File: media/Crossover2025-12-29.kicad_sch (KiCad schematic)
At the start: 11 parts, among them J1 GPIO, J2 Qwiic Right Angle, J3 Conn_01x04_Female, J4 Conn_01x03_Pin, J5 Conn_01x08_Socket, J6 Conn_01x02_Pin, J7 Screw_Terminal_01x02, Q1 2N4124

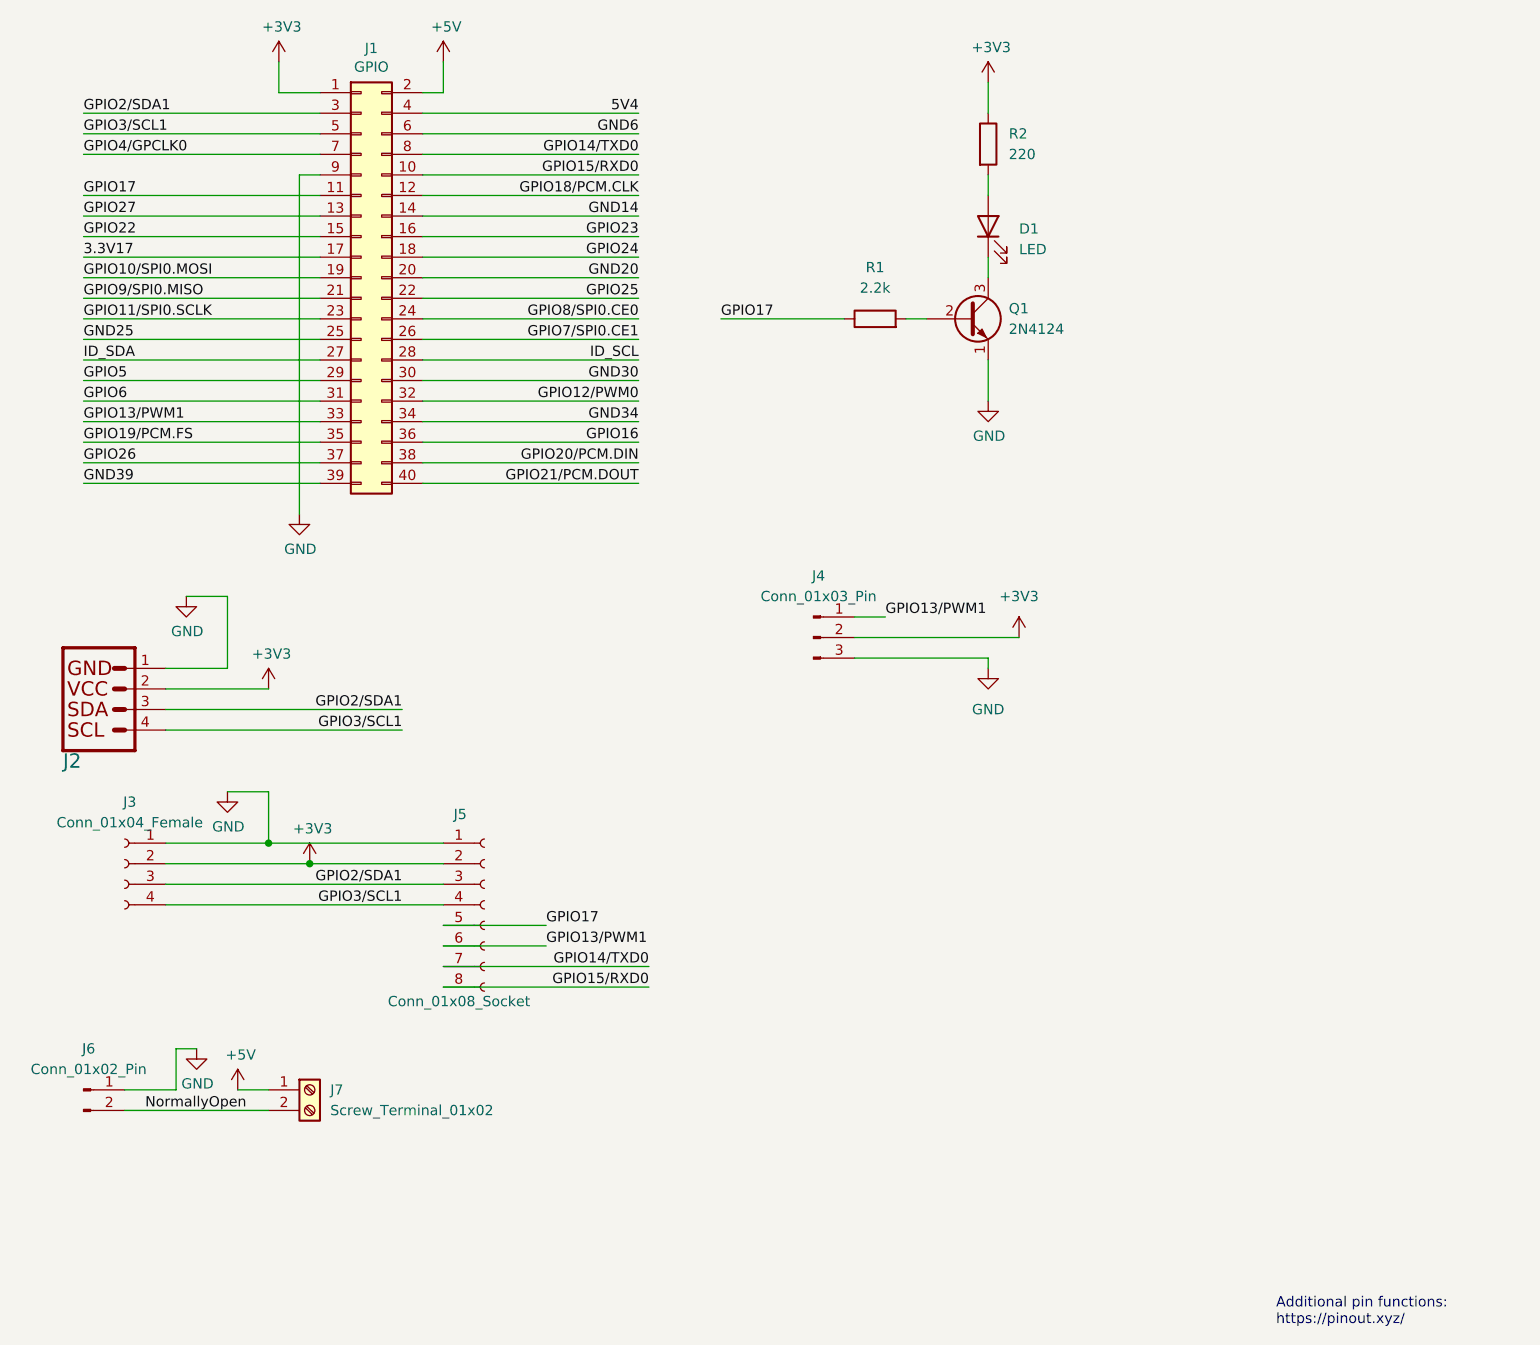
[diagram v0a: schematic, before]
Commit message: Add files via upload
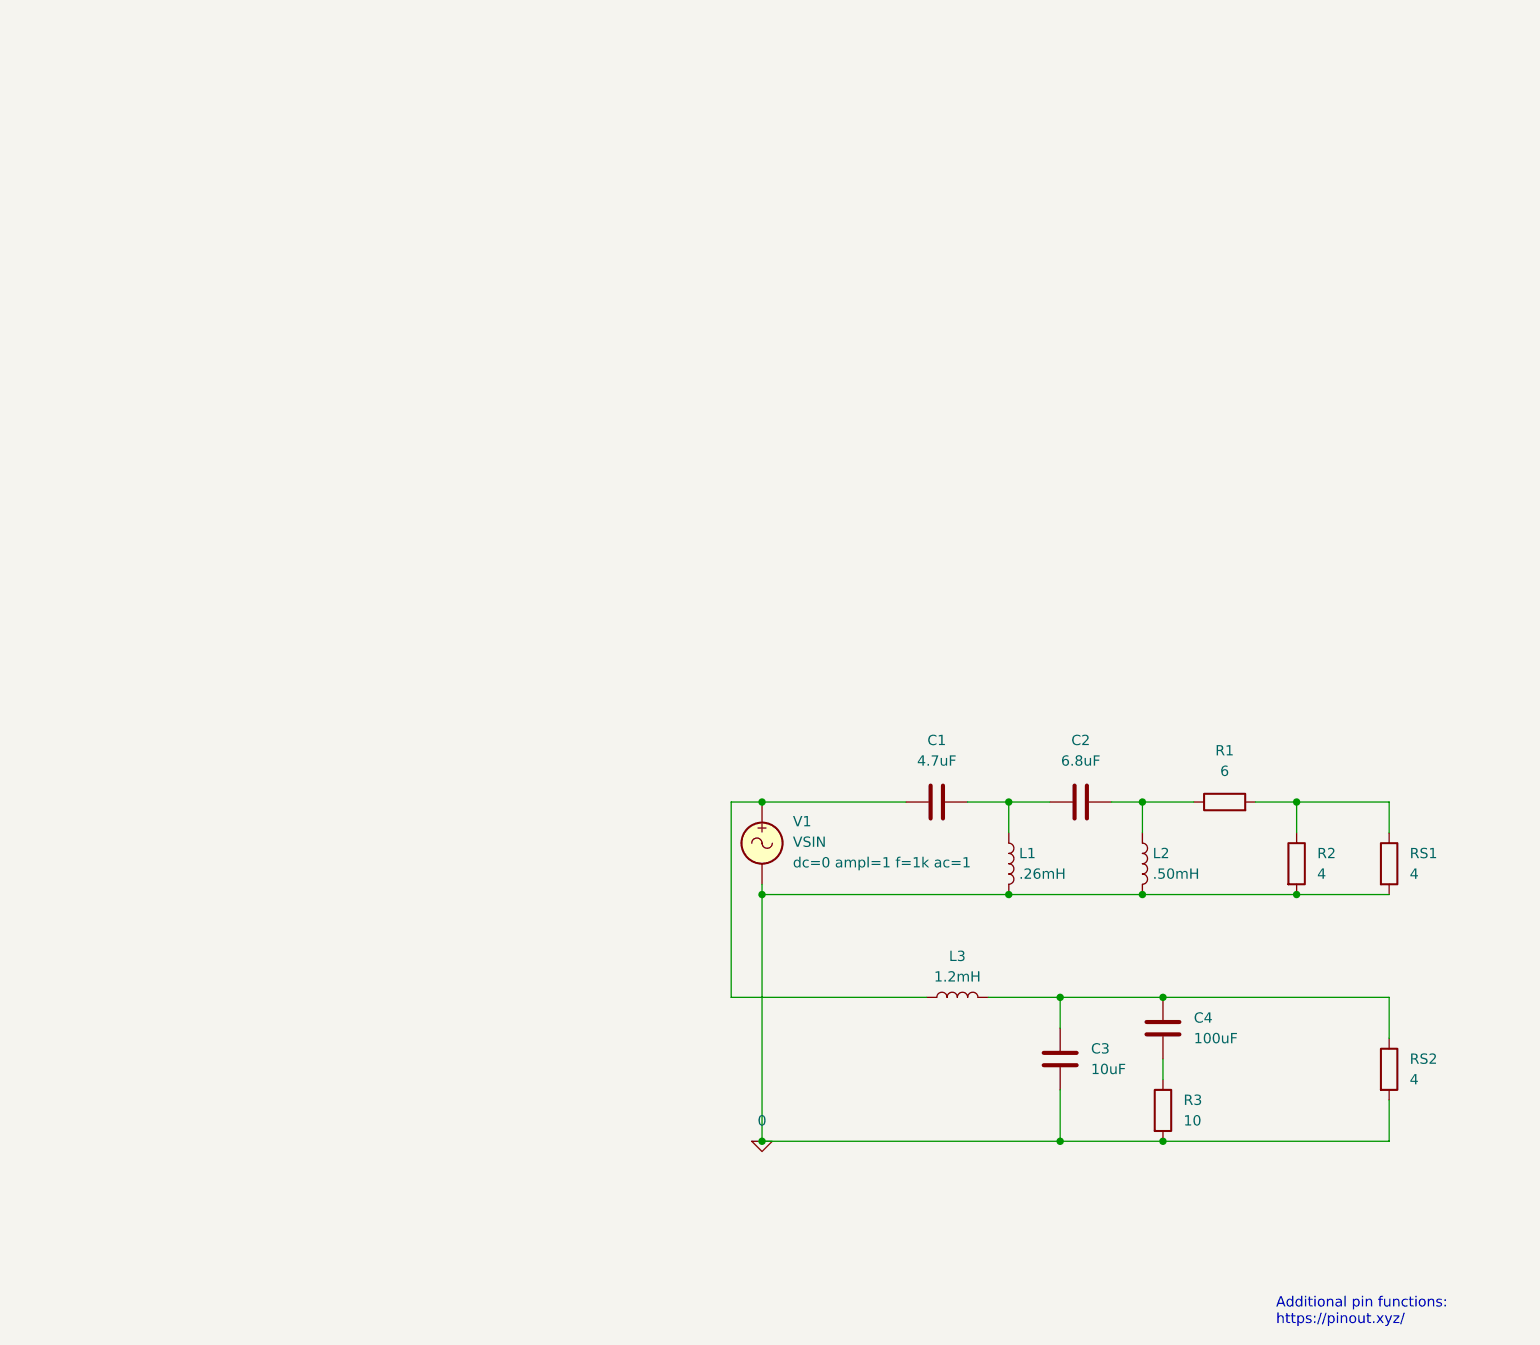
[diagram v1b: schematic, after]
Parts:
- removed D1: LED, LED_THT:LED_D5.0mm_Horizontal_O1.27mm_Z3.0mm, symbol Device:LED
- removed J1: GPIO, Connector_PinSocket_2.54mm:PinSocket_2x20_P2.54mm_Vertical, symbol Connector_Generic:Conn_02x20_Odd_Even
- removed J2: Qwiic Right Angle, Connector_PinSocket_2.00mm:PinSocket_1x04_P2.00mm_Horizontal, symbol Qwiic_pHat_for_Raspberry_Pi_v30-eagle-import:I2C_STANDARDQWIIC
- removed J3: Conn_01x04_Female, Connector_PinSocket_2.54mm:PinSocket_1x04_P2.54mm_Horizontal, symbol Connector:Conn_01x04_Female
- removed J4: Conn_01x03_Pin, Connector_PinHeader_2.54mm:PinHeader_1x03_P2.54mm_Horizontal, symbol Connector:Conn_01x03_Pin
- removed J5: Conn_01x08_Socket, Connector_PinSocket_2.54mm:PinSocket_1x08_P2.54mm_Horizontal, symbol Connector:Conn_01x08_Socket
- removed J6: Conn_01x02_Pin, Connector_JST:JST_PH_S2B-PH-K_1x02_P2.00mm_Horizontal, symbol Connector:Conn_01x02_Pin
- removed J7: Screw_Terminal_01x02, TerminalBlock_Phoenix:TerminalBlock_Phoenix_MPT-0,5-2-2.54_1x02_P2.54mm_Horizontal, symbol Connector:Screw_Terminal_01x02
- removed Q1: 2N4124, Package_TO_SOT_THT:TO-92_Inline_Wide, symbol Transistor_BJT:2N3904
- added C1: 4.7uF, symbol Device:C
- added C2: 6.8uF, symbol Device:C
- added C3: 10uF, symbol Device:C
- added C4: 100uF, symbol Device:C
- added L1: .26mH, symbol Device:L
- added L2: .50mH, symbol Device:L
- added L3: 1.2mH, symbol Device:L
- added R3: 10, Resistor_THT:R_Axial_DIN0207_L6.3mm_D2.5mm_P15.24mm_Horizontal, symbol Device:R
- added RS1, RS2: 4, Resistor_THT:R_Axial_DIN0207_L6.3mm_D2.5mm_P15.24mm_Horizontal, symbol Device:R
- added V1: VSIN, symbol Simulation_SPICE:VSIN
- R1: value 2.2k -> 6
- R2: value 220 -> 4
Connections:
- net +3V3 is gone; now on an unnamed net: R2.1
- net 0: now reaches R2.2
- net 0: now also C3.2, L1.2, L2.2, R3.2, RS1.2, RS2.2, V1.2
- net at R1.2: now also RS1.1
- net GPIO17: no longer names the net of R1.1
- net GPIO17: now also C2.2, L2.1
- new net: C3.1, C4.1, L3.2, RS2.1
- new net: C4.2, R3.1
- new net: C1.2, C2.1, L1.1
- new net: C1.1, L3.1, V1.1
